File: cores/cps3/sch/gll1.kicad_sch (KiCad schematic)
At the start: 1 part, among them J11 DL-3429-GLL1

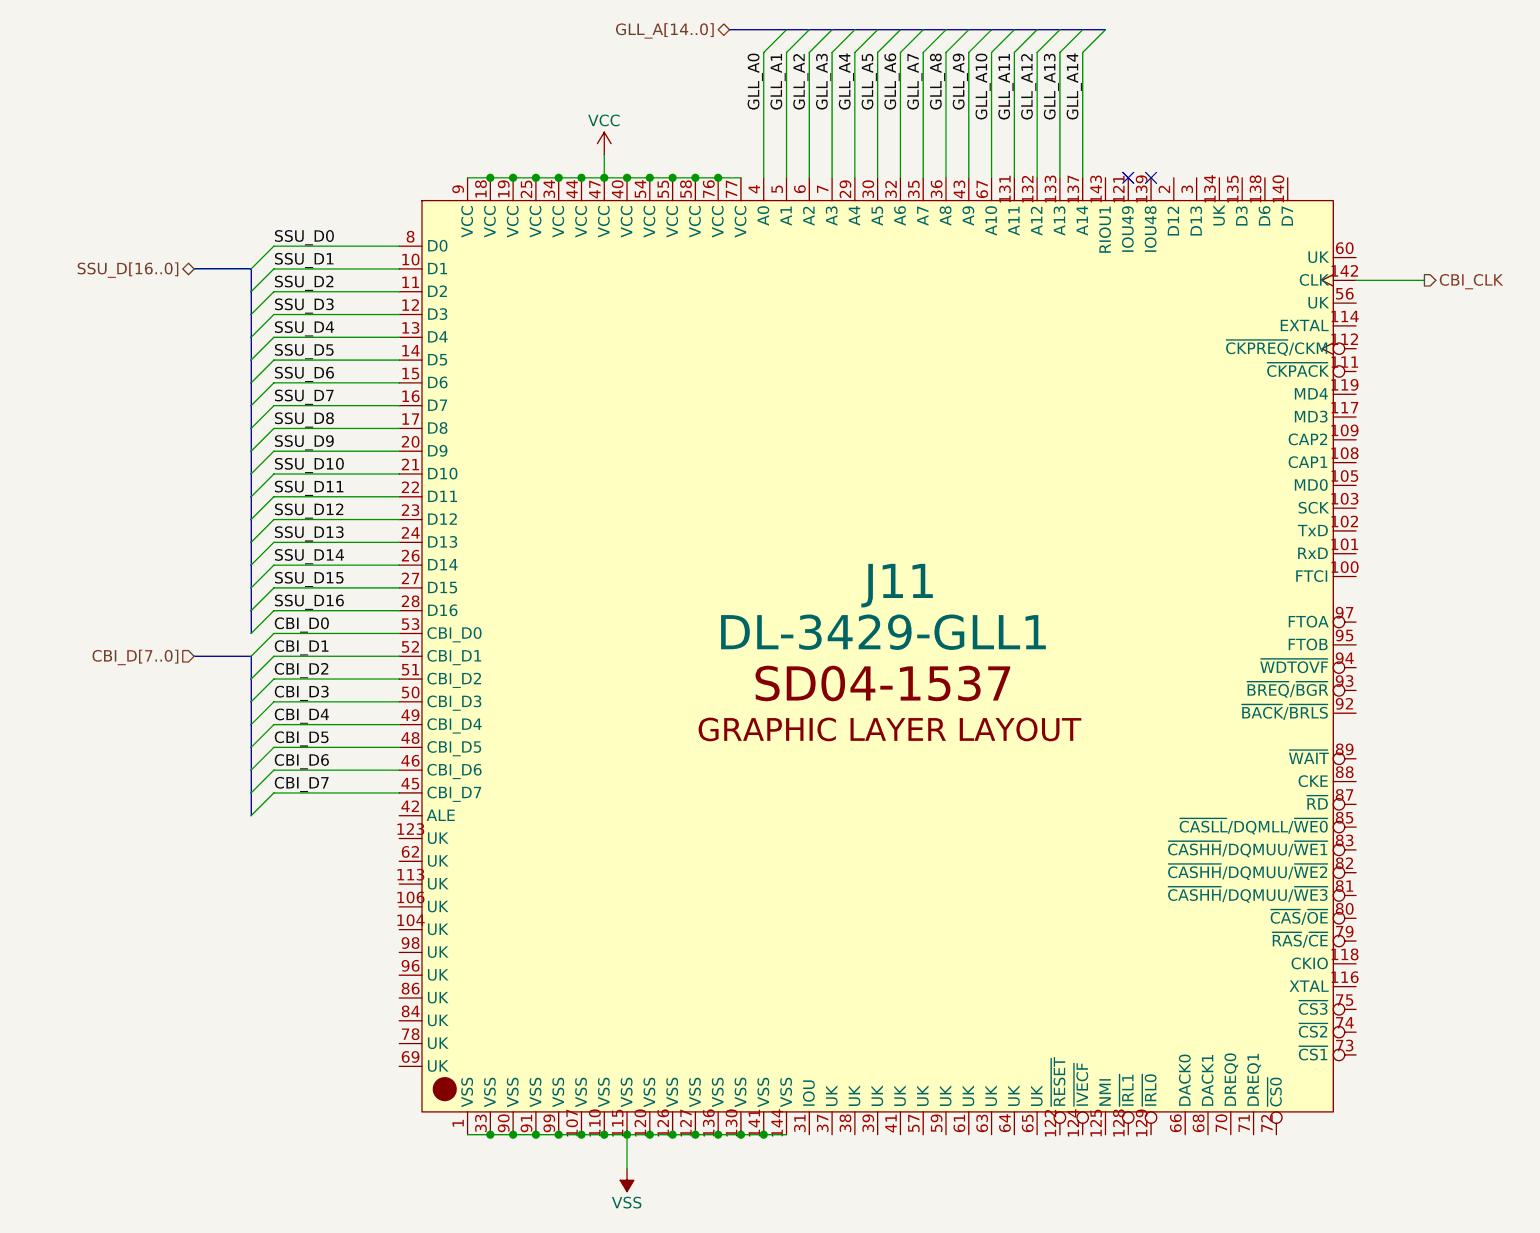
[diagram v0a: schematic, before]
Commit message: update_cps3
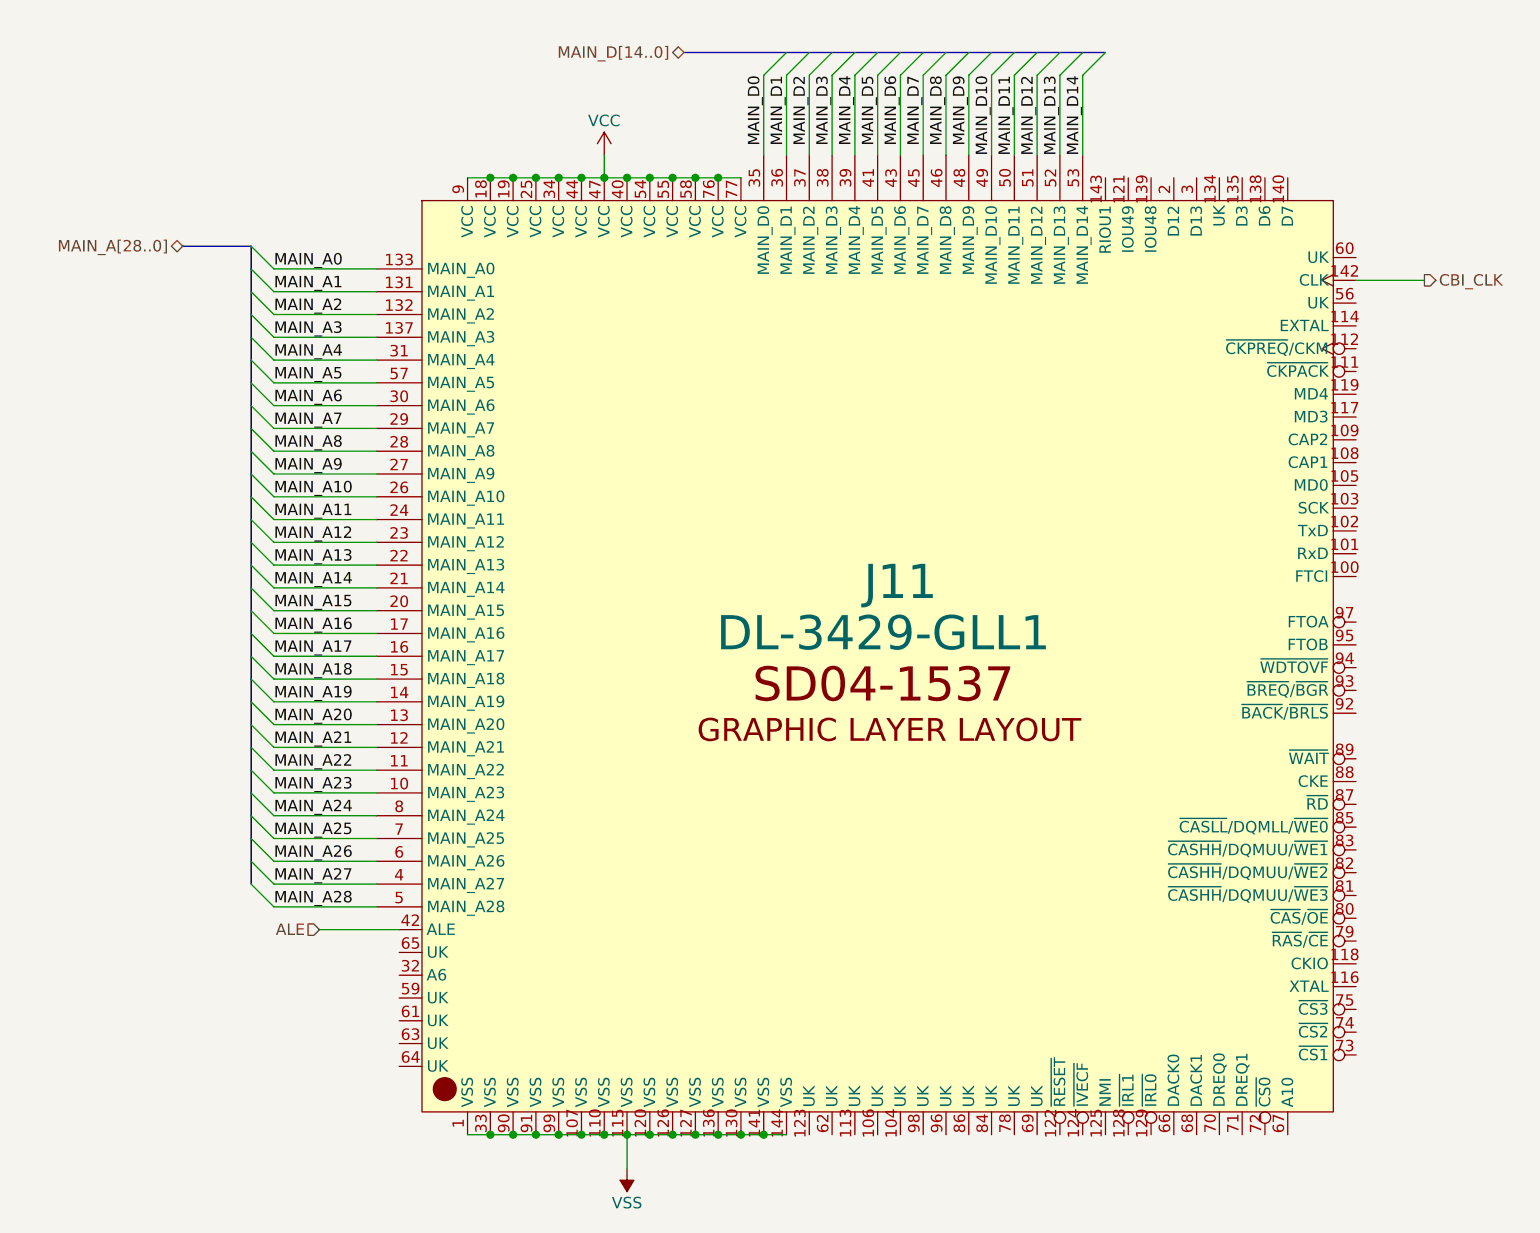
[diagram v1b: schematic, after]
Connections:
- net MAIN_A4: now reaches J11.31 (MAIN_A4)
- net MAIN_D2: now reaches J11.37 (MAIN_D2)
- net MAIN_D3: now reaches J11.38 (MAIN_D3)
- net MAIN_D4: now reaches J11.39 (MAIN_D4)
- net MAIN_D5: now reaches J11.41 (MAIN_D5)
- net ALE: now reaches J11.42 (ALE)
- net MAIN_A5: now reaches J11.57 (MAIN_A5)
- net CBI_D0 renamed MAIN_D14
- net CBI_D1 renamed MAIN_D13
- net CBI_D2 renamed MAIN_D12
- net CBI_D3 renamed MAIN_D11
- net CBI_D4 renamed MAIN_D10
- net CBI_D5 renamed MAIN_D9
- net CBI_D6 renamed MAIN_D8
- net CBI_D7 renamed MAIN_D7
- net GLL_A0 renamed MAIN_A27
- net GLL_A1 renamed MAIN_A28
- net GLL_A10: no longer names the net of J11.67 (A10)
- net GLL_A11 renamed MAIN_A1
- net GLL_A12 renamed MAIN_A2
- net GLL_A13 renamed MAIN_A0
- net GLL_A14 renamed MAIN_A3
- net GLL_A2 renamed MAIN_A26
- net GLL_A3 renamed MAIN_A25
- net GLL_A4 renamed MAIN_A7
- net GLL_A5 renamed MAIN_A6
- net GLL_A6: no longer names the net of J11.32 (A6)
- net GLL_A7 renamed MAIN_D0
- net GLL_A8 renamed MAIN_D1
- net GLL_A9 renamed MAIN_D6
- net SSU_D0 renamed MAIN_A24
- net SSU_D1 renamed MAIN_A23
- net SSU_D10 renamed MAIN_A14
- net SSU_D11 renamed MAIN_A13
- net SSU_D12 renamed MAIN_A12
- net SSU_D13 renamed MAIN_A11
- net SSU_D14 renamed MAIN_A10
- net SSU_D15 renamed MAIN_A9
- net SSU_D16 renamed MAIN_A8
- net SSU_D2 renamed MAIN_A22
- net SSU_D3 renamed MAIN_A21
- net SSU_D4 renamed MAIN_A20
- net SSU_D5 renamed MAIN_A19
- net SSU_D6 renamed MAIN_A18
- net SSU_D7 renamed MAIN_A17
- net SSU_D8 renamed MAIN_A16
- net SSU_D9 renamed MAIN_A15
- no-connect marks 2 -> 0
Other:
- moved on the sheet: J11
